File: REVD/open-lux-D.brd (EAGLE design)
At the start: 55.4 x 62 mm, 51 parts, among them IC2 MCP73831, IC3 ATMEGA32U4-AU, IC4 MCP1700-33, J1 AYZ0202, Q4 BSS123, T1 FDN340P, T2 FDN340P, X2 USBSMD, X3 8MHz

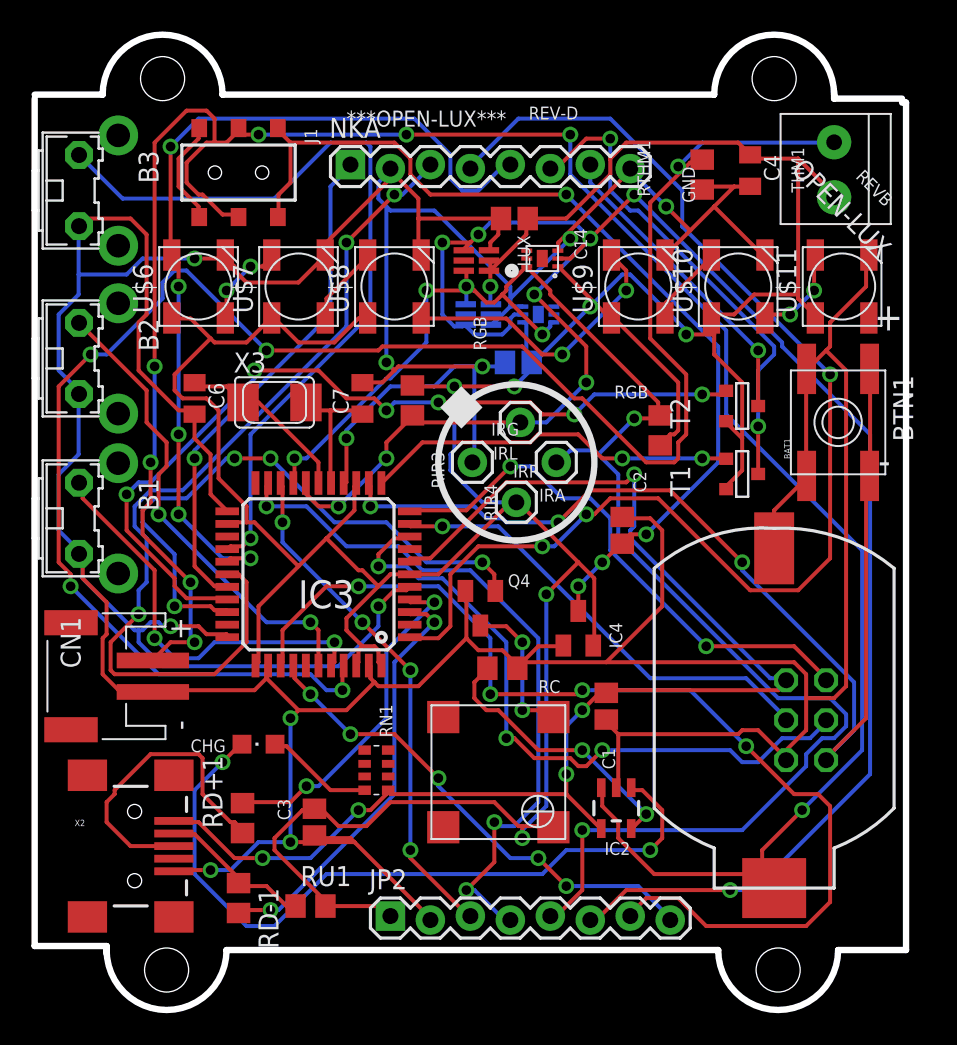
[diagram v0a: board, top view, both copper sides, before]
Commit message: update
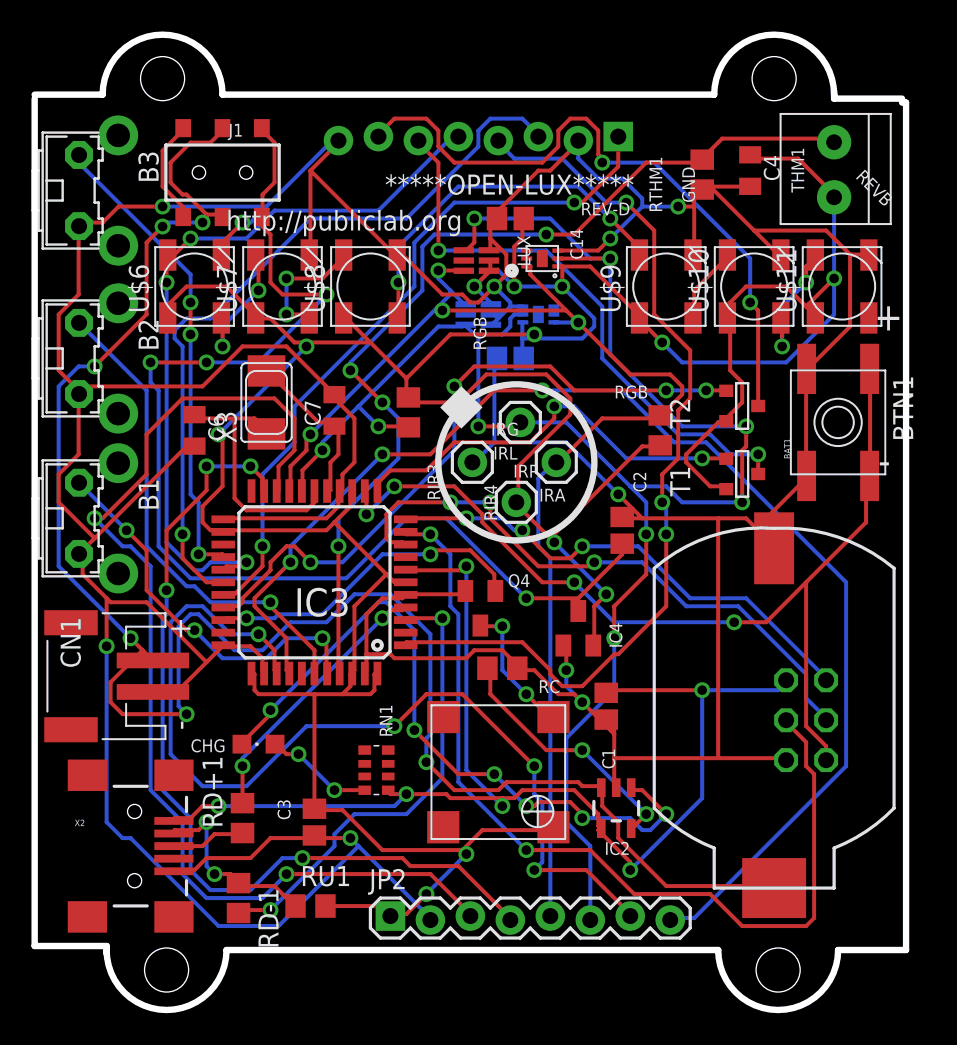
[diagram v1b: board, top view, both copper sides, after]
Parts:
- moved NKA 17.1 mm to (36.8, 51.3), flipped to the bottom
- moved C6 2.03 mm to (9.91, 32.8)
- moved C7 1.93 mm to (18.8, 34.0)
- moved U$9 1.78 mm to (39.9, 41.9)
- moved U$8 1.52 mm to (21.1, 41.9)
- moved U$7 1.02 mm to (15.5, 41.9)
- moved J1 1.02 mm to (11.7, 49.1)
- moved U$10 1.02 mm to (45.5, 41.9)
- moved RIR3 0.80 mm to (23.5, 33.9)
- moved IC3 0.57 mm to (17.5, 23.1)
- moved C5 0.57 mm to (30.0, 37.3)
- moved X3 0.51 mm to (14.5, 34.5), turned to 90 degrees
- moved U$6 0.25 mm to (9.91, 41.9)
- moved C14 0.25 mm to (30.0, 46.2)
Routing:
- net A5: track 115.9 -> 61.3 mm, vias 5 -> 4
- net A1: track 31.5 -> 81.4 mm, vias 5 -> 3
- net RXD: track 32.7 -> 68.9 mm, vias 4 -> 2
- net VBAT: track 148.1 -> 116.7 mm, vias 8 -> 6
- net GND: track 390.9 -> 361.8 mm, vias 11 -> 10
- net MOSI: track 29.2 -> 58.1 mm, vias 1 -> 2
- net N$4: track 19.8 -> 42.0 mm, vias 1 -> 2
- net D7: track 79.6 -> 58.1 mm
- net D12: track 51.0 -> 30.2 mm, vias 1 -> 3
- net SDA: track 105.3 -> 84.6 mm, vias 6 -> 4
- net D5: track 38.3 -> 20.8 mm, vias 4 -> 2
- net VDD: track 60.6 -> 76.0 mm
- net D+: track 19.8 -> 4.74 mm
- net SCL: track 129.4 -> 116.8 mm
- net D9: track 32.2 -> 44.7 mm, vias 1 -> 2
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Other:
- board text added: "*****OPEN-LUX*****"
- board text added: "http://publiclab.org"
- board text removed: "***OPEN-LUX***"
- board text removed: "OPEN-LUX"
